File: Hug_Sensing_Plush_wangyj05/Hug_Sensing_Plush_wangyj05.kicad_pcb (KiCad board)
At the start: 2 copper layers, 100 x 100 mm, 62 parts, among them J1 USB_C_Receptacle_USB2.0_16P, J2 Header B2B-PH-SM4-TBLFSN, SW1 SW_SPST, SW2 SW_SPST, U1 BQ24040DSQR, U2 TPS63802DLAR, U3 ESP32-S3-WROOM-1-N4, U4 DRV2605LDGS, U5 USBLC6-2SC6, U6 MPRLS0025PA00001A

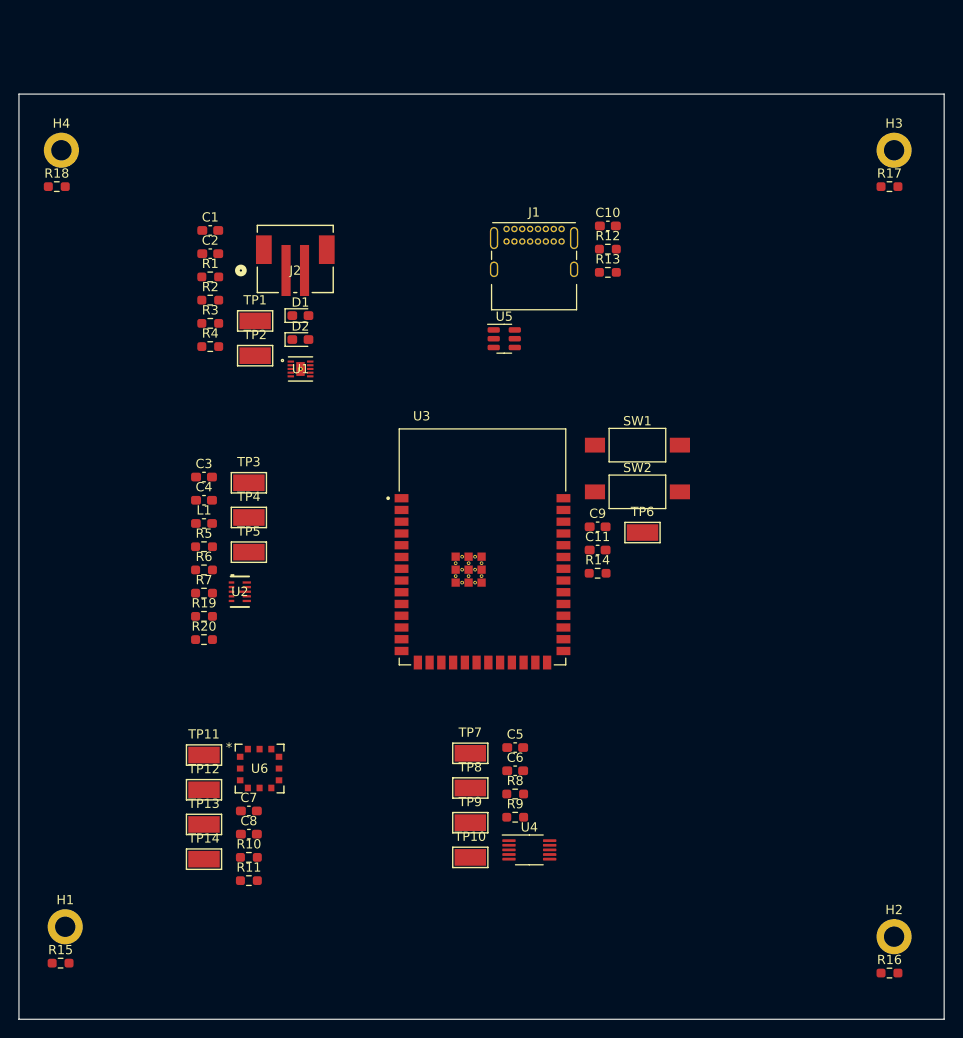
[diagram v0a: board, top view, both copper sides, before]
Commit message: Edited board layout
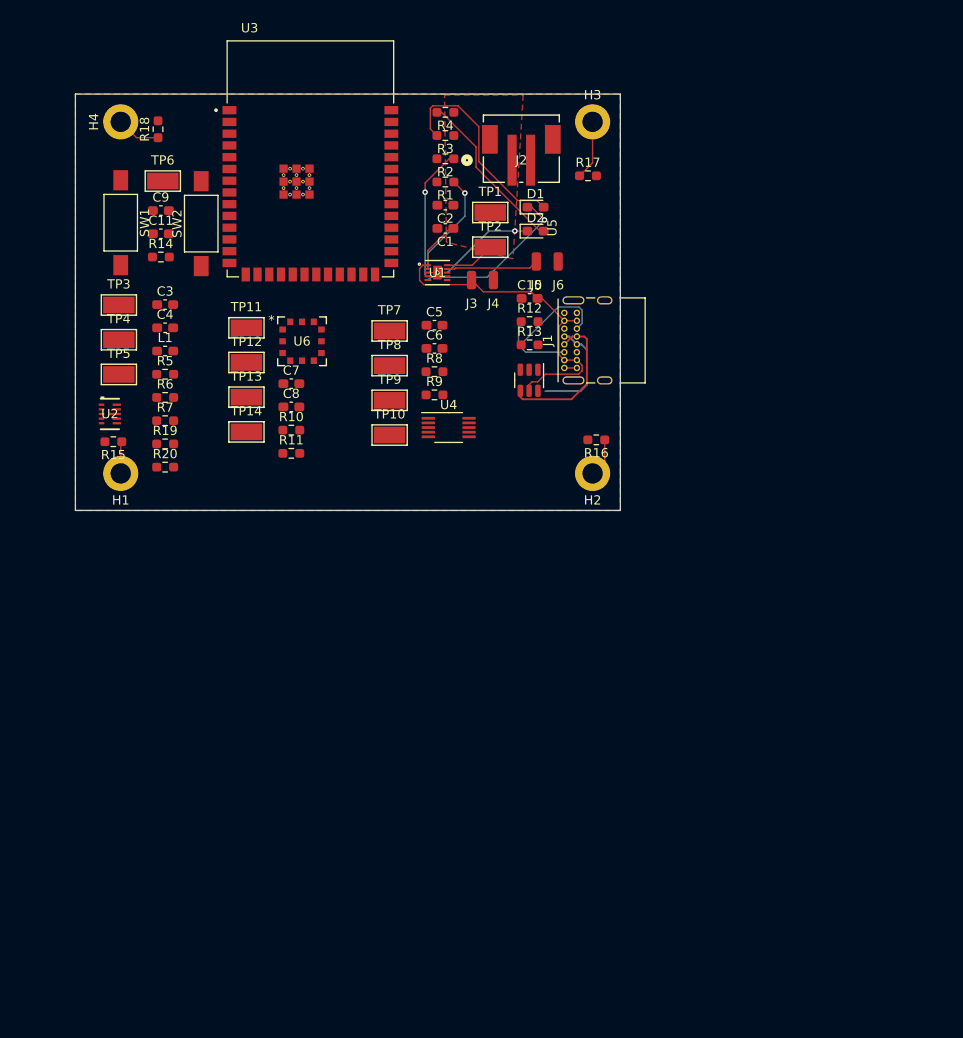
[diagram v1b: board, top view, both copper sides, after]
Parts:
- added J3: Wire Pad, Connector_Wire:SolderWirePad_1x01_SMD_1x2mm, F.Cu at (93.9, 55.1)
- added J4: Wire Pad, Connector_Wire:SolderWirePad_1x01_SMD_1x2mm, F.Cu at (96.3, 55.1)
- added J5: Wire Pad, Connector_Wire:SolderWirePad_1x01_SMD_1x2mm, F.Cu at (100.9, 53.1)
- added J6: Wire Pad, Connector_Wire:SolderWirePad_1x01_SMD_1x2mm, F.Cu at (103.3, 53.1)
- moved R16 65.8 mm to (107.4, 72.4), turned to 180 degrees
- moved TP6 64.3 mm to (60.5, 44.4)
- moved SW1 60.8 mm to (56.0, 48.9), turned to -90 degrees
- moved H2 59.7 mm to (107.0, 76.0), turned to 180 degrees
- moved R14 58.3 mm to (60.3, 52.6)
- moved C11 58.3 mm to (60.3, 50.1)
- moved C9 58.3 mm to (60.3, 47.6)
- moved R15 56.6 mm to (55.2, 72.6), turned to 180 degrees
- moved SW2 55.3 mm to (64.7, 49.0), turned to 90 degrees
- moved H1 49.4 mm to (56.0, 76.0), turned to 180 degrees
- moved R8 46.5 mm to (89.9, 65.0)
- moved TP10 46.5 mm to (85.1, 71.8)
- moved TP8 46.5 mm to (85.1, 64.3)
- moved TP9 46.5 mm to (85.1, 68.1)
- moved C5 46.5 mm to (89.9, 60.0)
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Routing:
- net +5V: track 0.00 -> 41.4 mm
- net Net-(D1-A): track 0.00 -> 22.4 mm
- net Net-(D1-K): track 0.00 -> 18.2 mm, vias 0 -> 1
- net Net-(D2-A): track 0.00 -> 18.1 mm
- net /USB-C Connector/D+: track 0.00 -> 16.4 mm
- net Net-(U1-PRETERM): track 0.00 -> 14.4 mm, vias 0 -> 1
- net /USB-C Connector/D-: track 0.00 -> 11.6 mm
- net Net-(U1-ISET): track 0.00 -> 11.6 mm, vias 0 -> 1
- net Net-(J1-CC2): track 0.00 -> 10.6 mm
- net Net-(D2-K): track 0.00 -> 10.5 mm, vias 0 -> 1
- net /Battery and Battery Charger/TS: track 0.00 -> 9.97 mm
- net Net-(J1-CC1): track 0.00 -> 7.83 mm
- net Net-(H3-Pad1): track 0.00 -> 6.42 mm
- net Battery_3V_4V2: track 0.00 -> 5.47 mm
- net Net-(H4-Pad1): track 0.00 -> 4.74 mm
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- added copper zone on F.Cu, net Battery_3V_4V2
- added copper zone on F.Cu, net GND
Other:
- board size 100 x 100 mm -> 58.9 x 45 mm
- board text removed: "Battery charger"
- board text removed: "Buck-boost converter"
- board text removed: "ESP32"
- board text removed: "Motor Driver"
- board text removed: "Pressure sensor"
- board text removed: "USB-C"
